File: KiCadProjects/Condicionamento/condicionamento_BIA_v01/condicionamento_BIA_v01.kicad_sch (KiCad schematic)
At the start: 34 parts, among them J1 Vref, J2 tensoes, J3 sinais analogicos, J4 comunicacao / sinais digitais, U1 AD828AN, U2 AD828AN

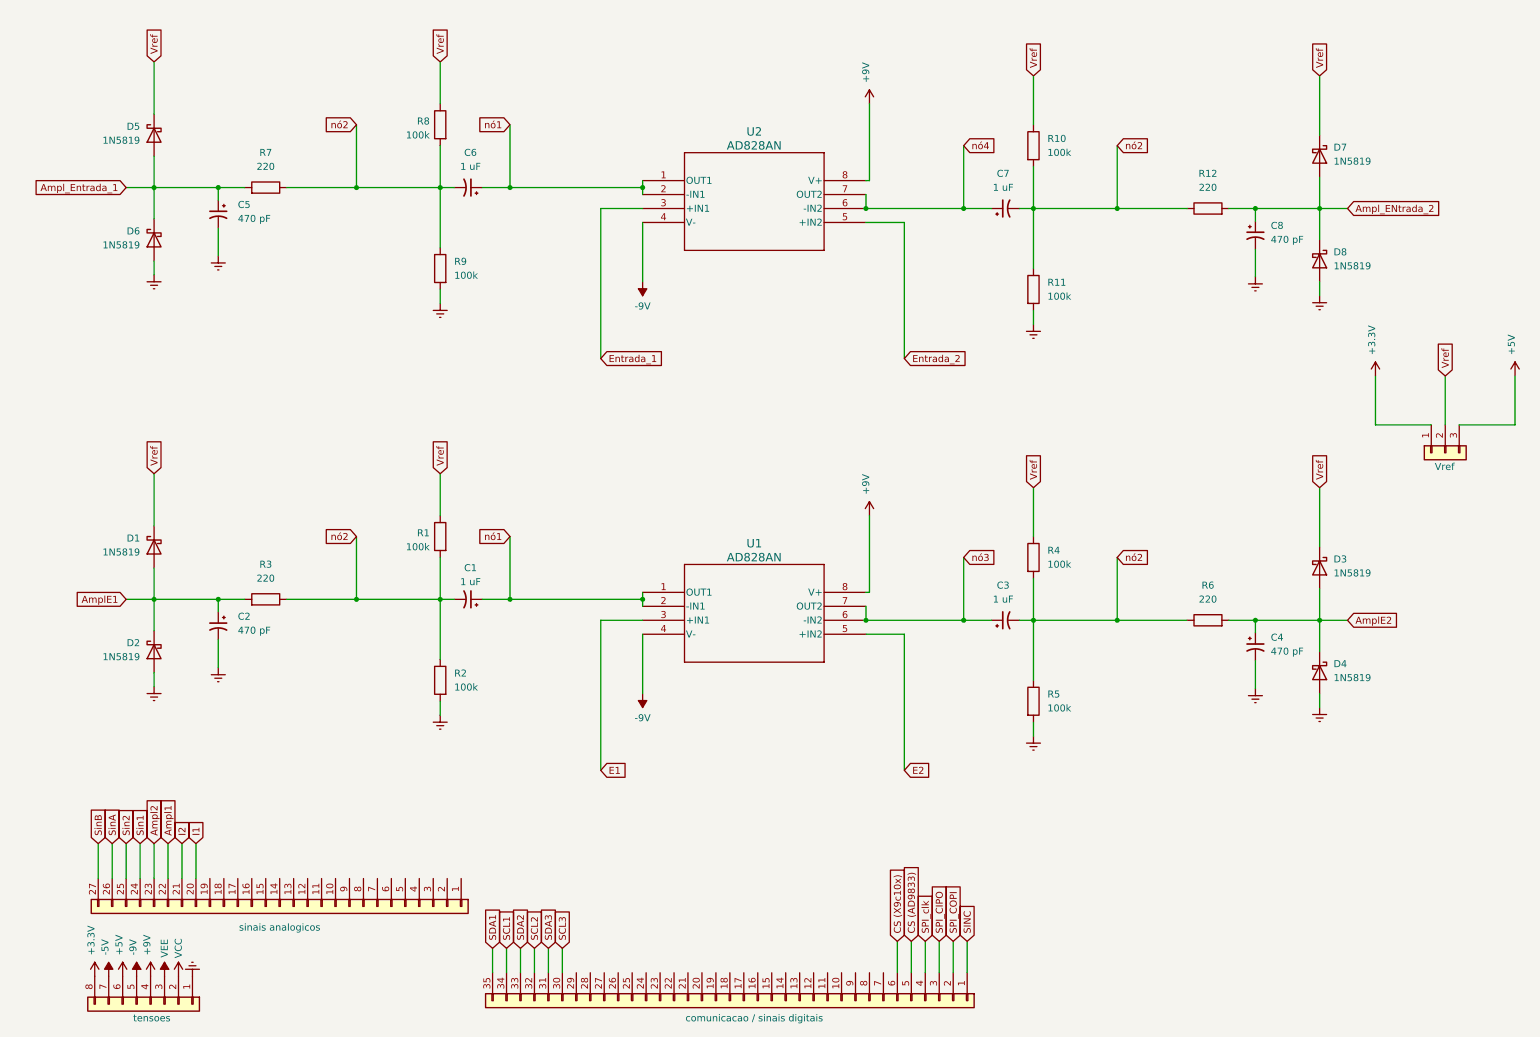
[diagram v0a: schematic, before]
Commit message: reposicionamento do circuito
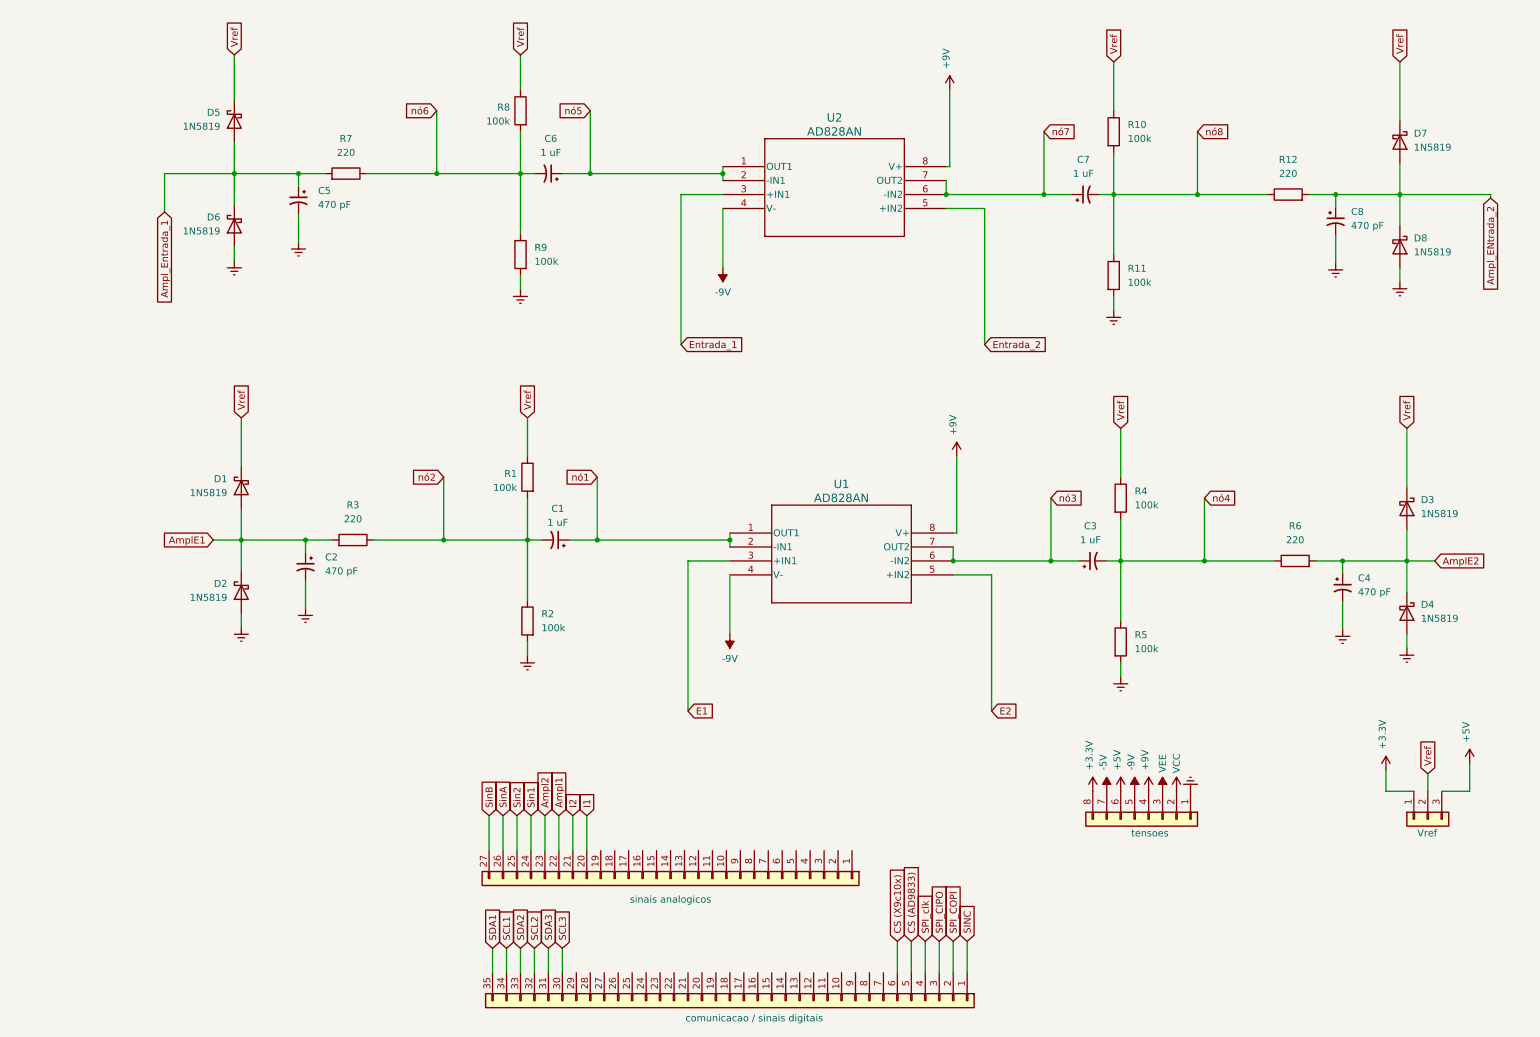
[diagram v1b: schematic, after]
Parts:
- U1, U2: footprint N_8_ADI -> AD828AN:N_8_ADI
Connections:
- net nó1: no longer C6.1, U2.1 (OUT1), U2.2 (-IN1)
- net nó2: no longer C3.2, C6.2, C7.2, R10.2, R11.1, R12.1, R4.2, R5.1, R6.1, R7.1, R8.2, R9.1
- net nó4: now also C3.2, R4.2, R5.1, R6.1; no longer C7.1, U2.6 (-IN2), U2.7 (OUT2)
- new net nó5: C6.1, U2.1 (OUT1), U2.2 (-IN1)
- new net nó6: C6.2, R7.1, R8.2, R9.1
- new net nó7: C7.1, U2.6 (-IN2), U2.7 (OUT2)
- new net nó8: C7.2, R10.2, R11.1, R12.1
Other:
- moved on the sheet: C1, C2, C3, C4, C5, C6, C7, C8, D1, D2, D3, D4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

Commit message: condicionamento
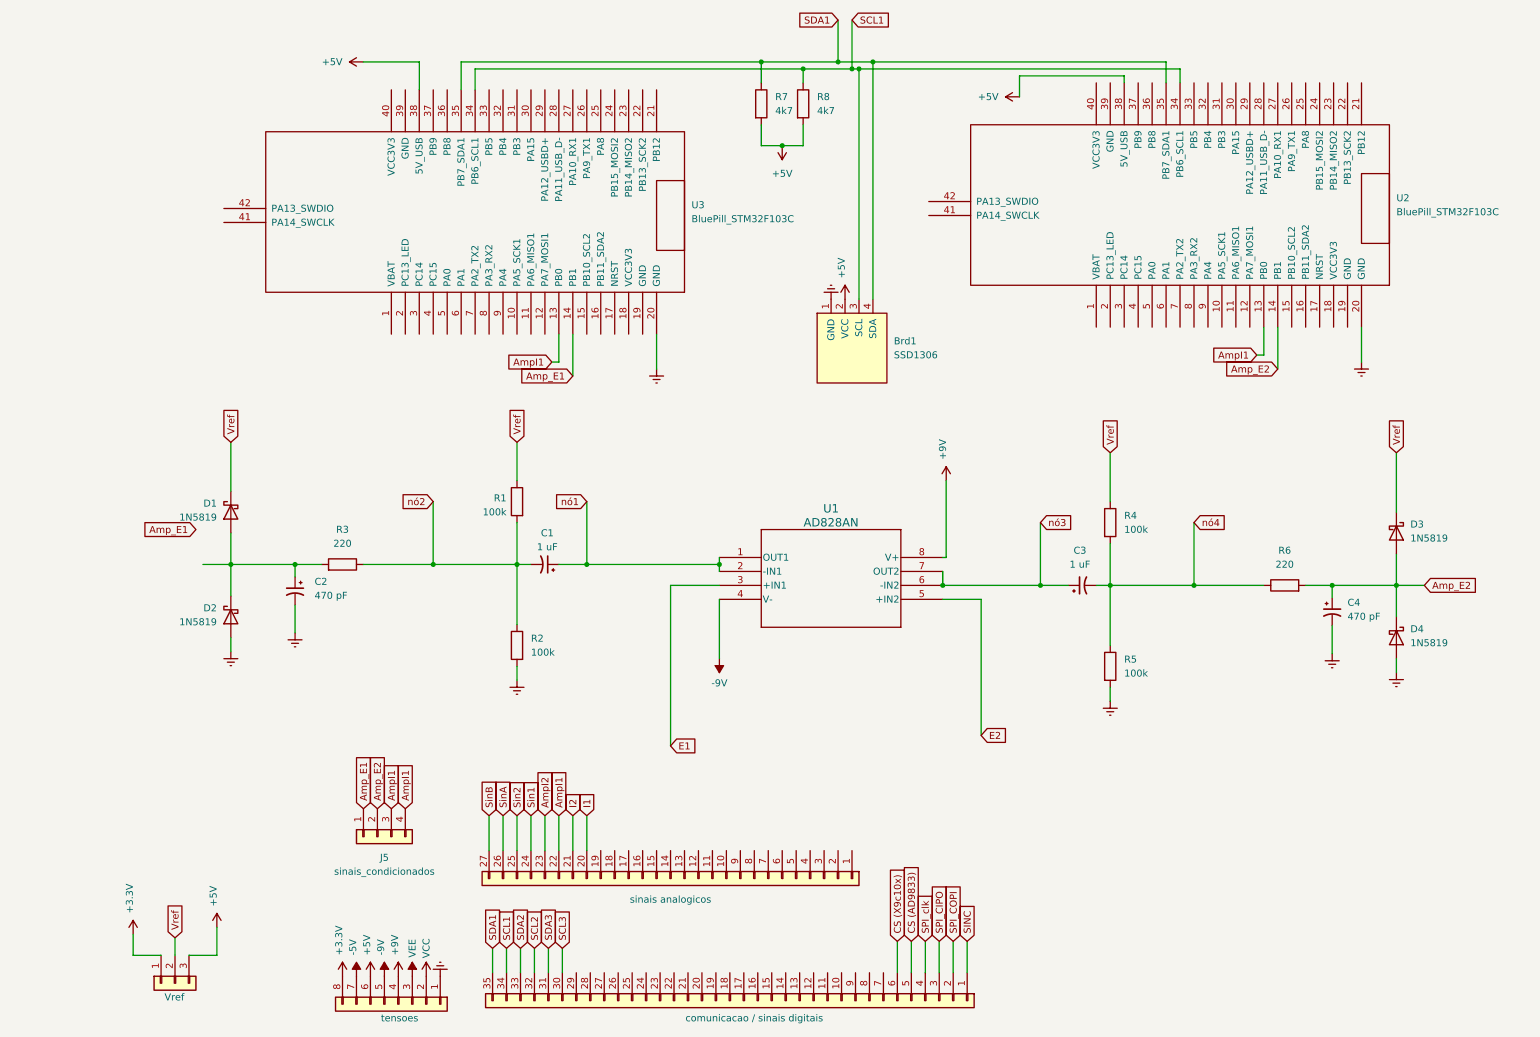
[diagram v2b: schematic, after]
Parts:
- removed C5, C8: 470 pF, Capacitor_THT:CP_Radial_D5.0mm_P2.50mm, symbol Device:C_Polarized_Small_US
- removed C6, C7: 1 uF, Capacitor_THT:CP_Radial_D5.0mm_P2.50mm, symbol Device:C_Polarized_Small_US
- removed D5, D6, D7, D8: 1N5819, Diode_THT:D_DO-41_SOD81_P10.16mm_Horizontal, symbol Diode:1N5819
- removed R10, R11, R9: 100k, Resistor_THT:R_Axial_DIN0207_L6.3mm_D2.5mm_P7.62mm_Horizontal, symbol Device:R
- removed R12: 220, Resistor_THT:R_Axial_DIN0207_L6.3mm_D2.5mm_P7.62mm_Horizontal, symbol Device:R
- removed U2: AD828AN, AD828AN:N_8_ADI, symbol AD828AN:AD828AN
- added Brd1: SSD1306, SSD1306:128x64OLED, symbol SSD1306-128x64_OLED:SSD1306
- added J5: sinais_condicionados, Connector_PinHeader_2.54mm:PinHeader_1x04_P2.54mm_Horizontal, symbol Connector_Generic:Conn_01x04
- added U2, U3: BluePill_STM32F103C, BluePill_breakouts:BluePill_STM32F103C, symbol bluepill_breakouts:BluePill_STM32F103C
- R7: value 220 -> 4k7
- R8: value 100k -> 4k7
- U1: footprint AD828AN:N_8_ADI -> footprints:N_8_ADI
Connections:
- net Ampl_Entrada_1 is gone; now on net +5V: R7.2
- net +5V: now also R8.2, Brd1.2 (VCC), U2.38 (5V_USB), U3.38 (5V_USB)
- net Earth: now also Brd1.1 (GND), U2.20 (GND), U3.20 (GND)
- net SCL1: now also R8.1, Brd1.3 (SCL), U2.34 (PB6_SCL1), U3.34 (PB6_SCL1)
- net SDA1: now also R7.1, Brd1.4 (SDA), U2.35 (PB7_SDA1), U3.35 (PB7_SDA1)
- net Vref: no longer R8.1
- net Ampl1 renamed AmpI1
- net AmpI1: now also J5.3 (Pin_3), J5.4 (Pin_4), U2.13 (PB0), U3.13 (PB0)
- net Ampl2 renamed AmpI2
- net AmplE1: no longer names the net of C2.1, D1.2 (A), D2.1 (K), R3.2
- net AmplE2 renamed Amp_E2
- net Amp_E2: now also J5.2 (Pin_2), U2.14 (PB1)
- removed net nó6: R7.1, R8.2
- new net Amp_E1: J5.1 (Pin_1), U3.14 (PB1)
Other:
- moved on the sheet: C1, C2, C3, C4, D1, D2, D3, D4, R1, R2, R3, R4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
